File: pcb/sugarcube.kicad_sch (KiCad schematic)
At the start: 23 parts, among them J1 SIM_Card, J2 USB_C_Receptacle_USB2.0_14P, J3 Conn_01x02, U1 nRF9151-LAXX, U2 nPM1300-QEXX

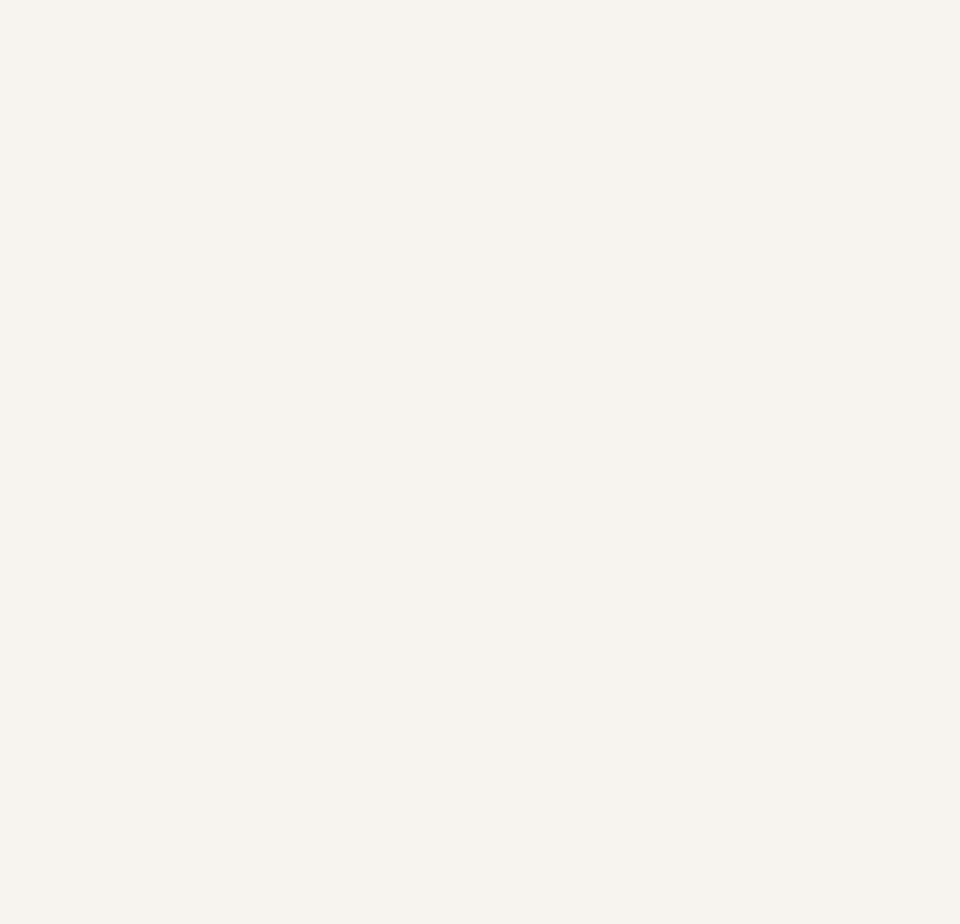
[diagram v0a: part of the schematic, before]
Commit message: epd driver
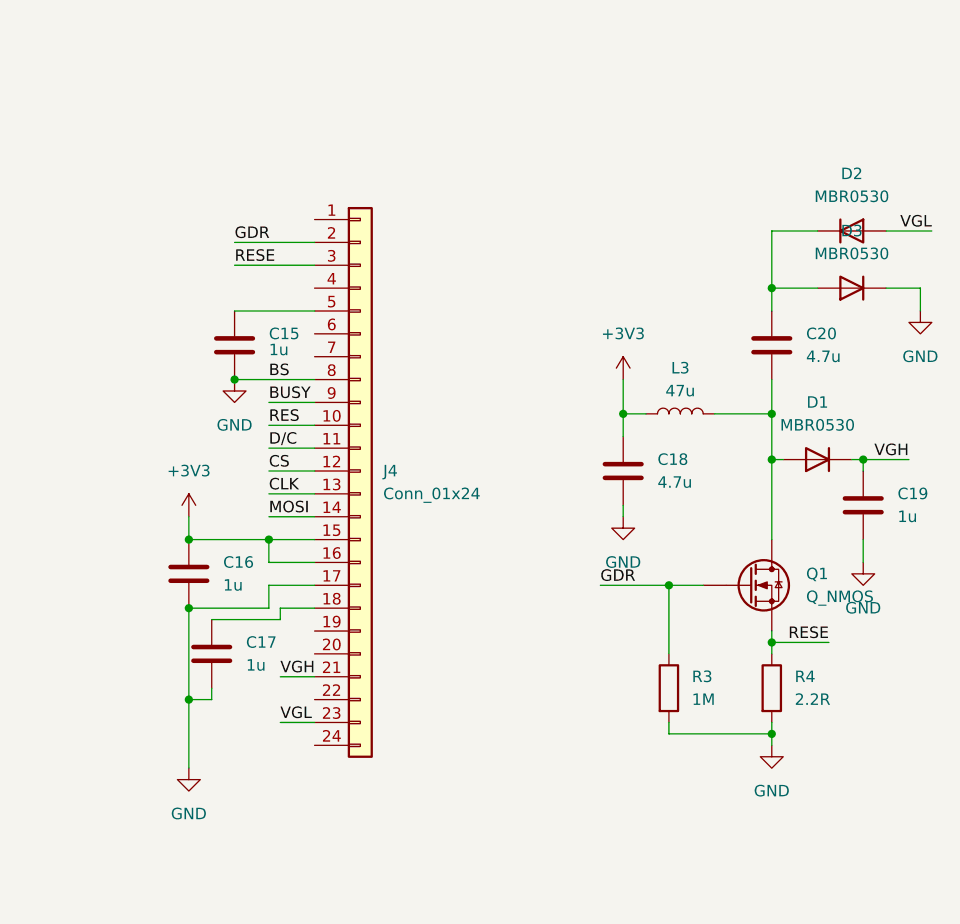
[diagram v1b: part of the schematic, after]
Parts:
- added C15, C16, C17, C19: 1u, symbol Device:C
- added C18, C20: 4.7u, symbol Device:C
- added D1, D2, D3: MBR0530, symbol Device:D
- added J4: Conn_01x24, symbol Connector_Generic:Conn_01x24
- added L3: 47u, symbol Device:L
- added Q1: Q_NMOS, symbol Device:Q_NMOS
- added R3: 1M, symbol Device:R
- added R4: 2.2R, symbol Device:R
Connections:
- net +3V3: now also C16.1, C18.1, J4.15 (Pin_15), J4.16 (Pin_16), L3.1
- net GND: now also C15.1, C16.2, C17.2, C18.2, C19.2, D3.1 (K), J4.17 (Pin_17), J4.8 (Pin_8), R3.2, R4.2
- new net: C20.1, D2.1 (K), D3.2 (A)
- new net: C20.2, D1.2 (A), L3.2, Q1.D
- new net: C17.1, J4.18 (Pin_18)
- new net: C15.2, J4.5 (Pin_5)
- new net BUSY: J4.9 (Pin_9)
- new net CLK: J4.13 (Pin_13)
- new net CS: J4.12 (Pin_12)
- new net D/C: J4.11 (Pin_11)
- new net GDR: J4.2 (Pin_2), Q1.G, R3.1
- new net MOSI: J4.14 (Pin_14)
- new net RES: J4.10 (Pin_10)
- new net RESE: J4.3 (Pin_3), Q1.S, R4.1
- new net VGH: C19.1, D1.1 (K), J4.21 (Pin_21)
- new net VGL: D2.2 (A), J4.23 (Pin_23)
